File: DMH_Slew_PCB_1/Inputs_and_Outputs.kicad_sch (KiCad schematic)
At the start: 25 parts, among them J1 TS_Jack_6.35mm_Sw, J10 TS_Jack_6.35mm_Sw, J11 TS_Jack_6.35mm_Sw, J2 TS_Jack_6.35mm_Sw, J200 IDC_02x05, J3 TS_Jack_6.35mm_Sw, J4 TS_Jack_6.35mm_Sw, J5 TS_Jack_6.35mm_Sw, J6 TS_Jack_6.35mm_Sw, J7 TS_Jack_6.35mm_Sw, J8 TS_Jack_6.35mm_Sw, J9 TS_Jack_6.35mm_Sw, U1 TL074, U2 TL072

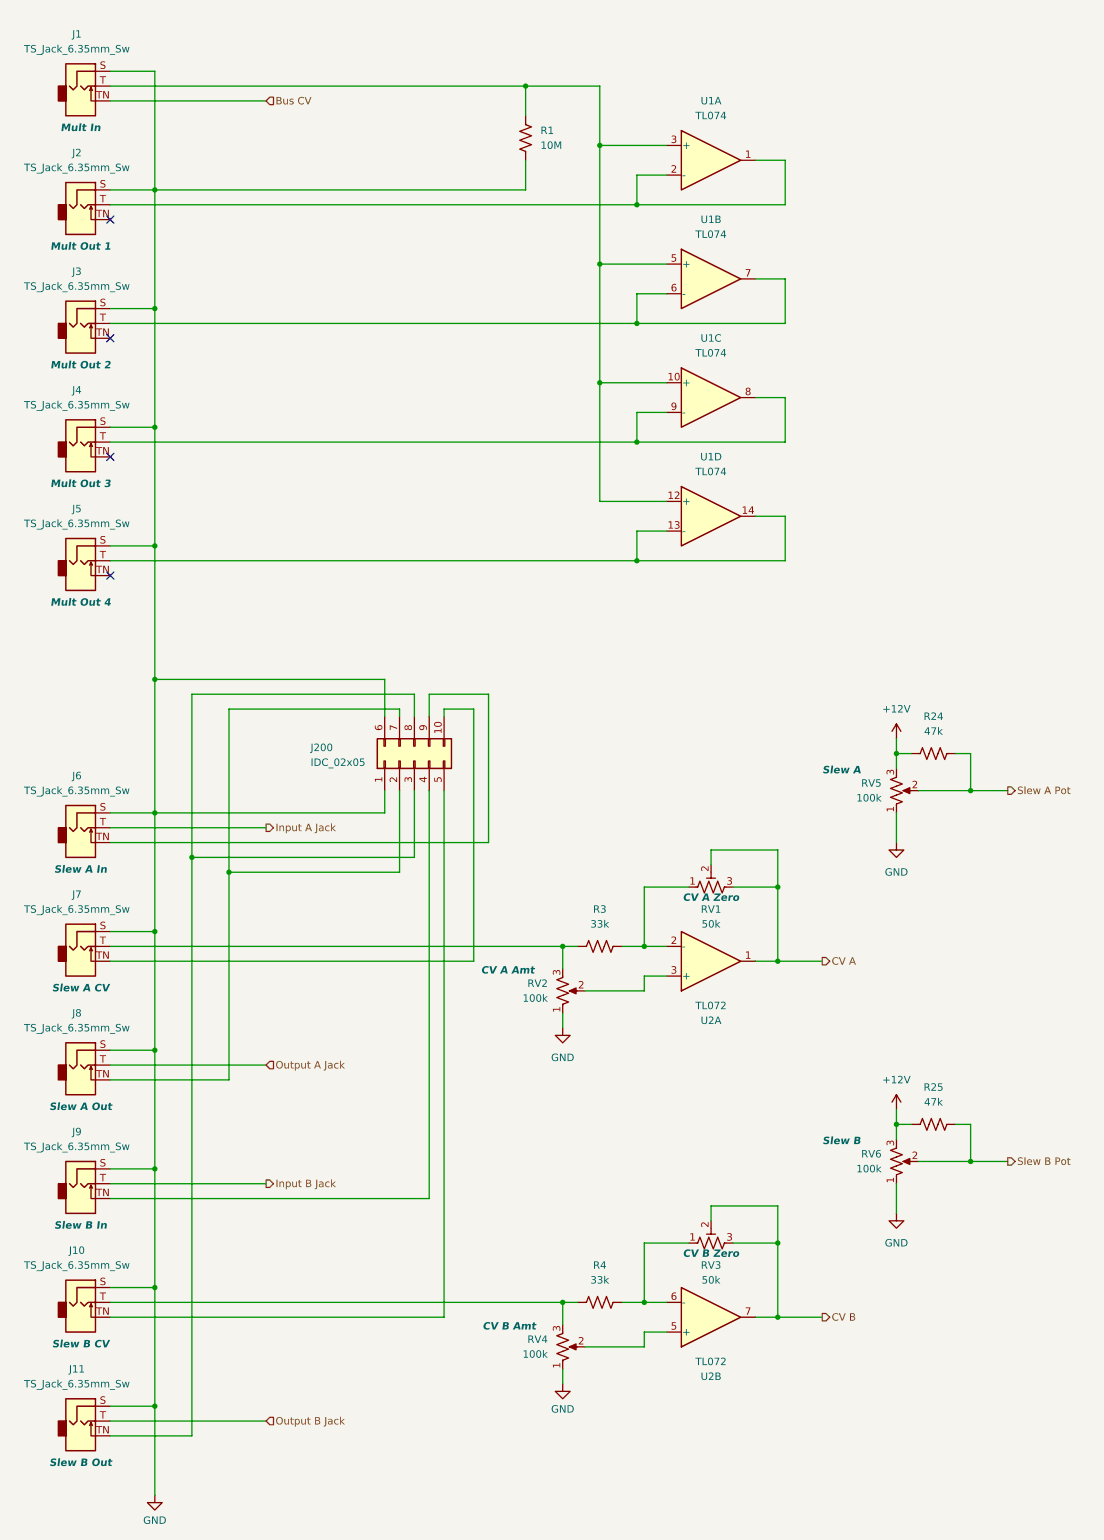
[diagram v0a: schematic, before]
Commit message: Schematic design in progress
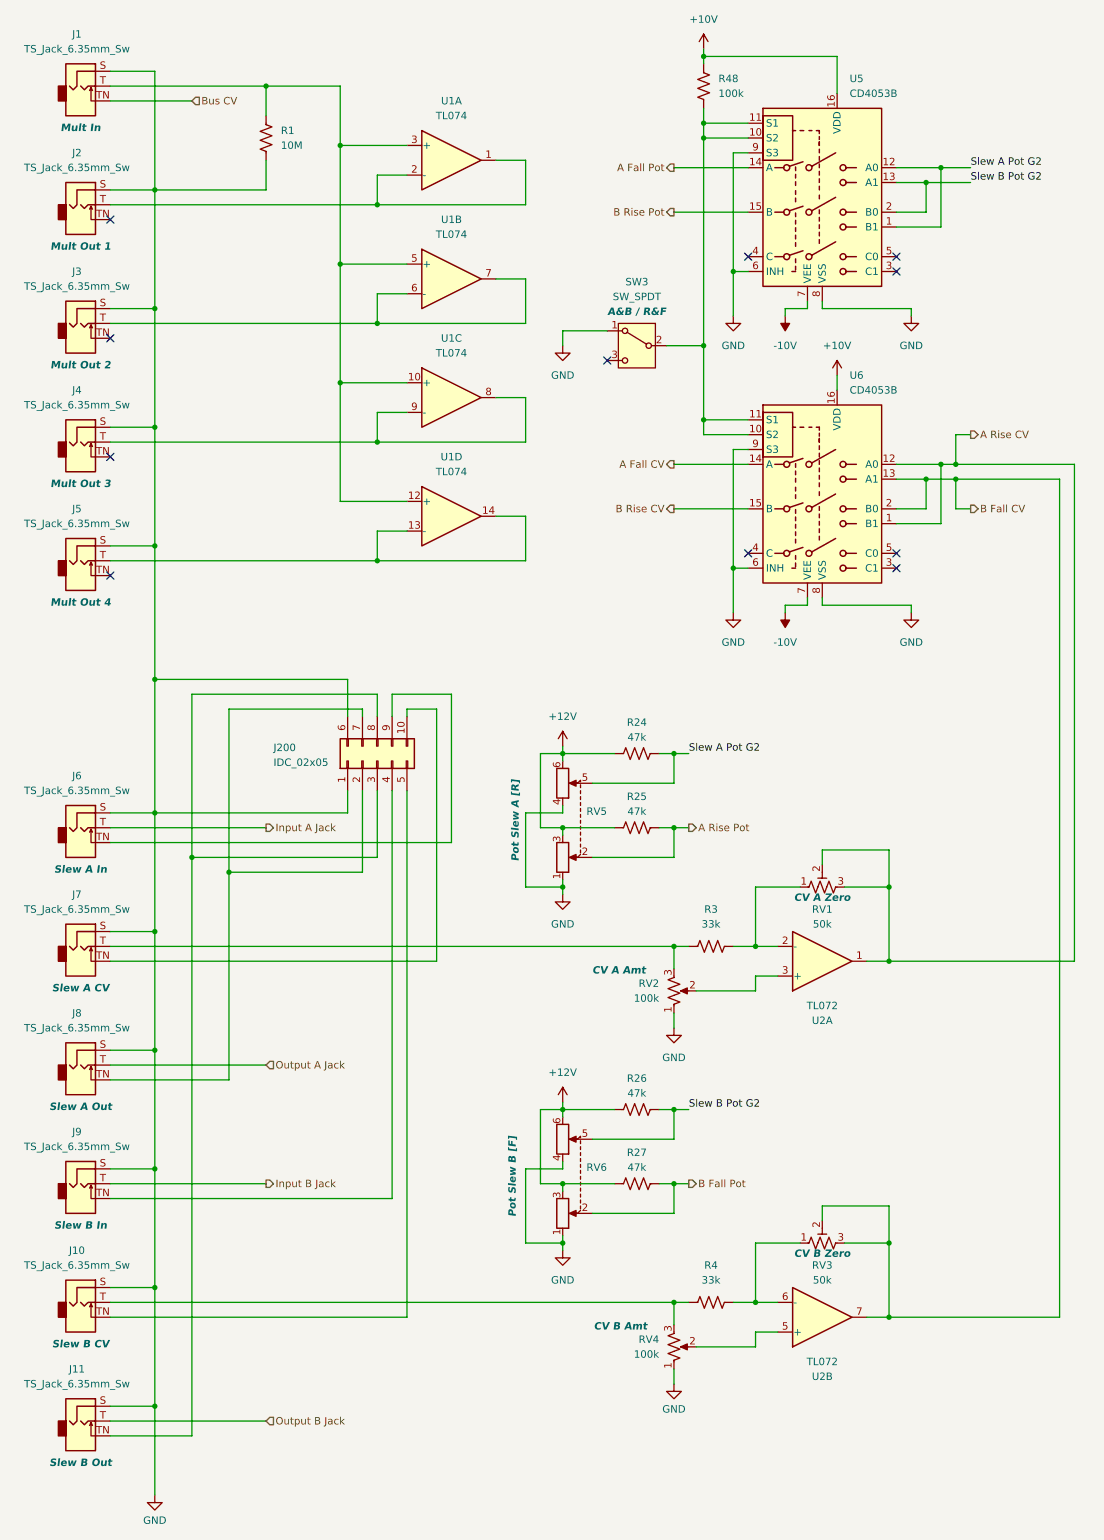
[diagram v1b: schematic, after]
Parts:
- removed RV5, RV6: 100k, SynthStuff:Potentiometer_TT_P110KH1, symbol Device:R_Potentiometer_US
- added R26, R27: 47k, Resistor_THT:R_Axial_DIN0207_L6.3mm_D2.5mm_P7.62mm_Horizontal, symbol Device:R_US
- added R48: 100k, Resistor_THT:R_Axial_DIN0207_L6.3mm_D2.5mm_P7.62mm_Horizontal, symbol Device:R_US
- added RV5, RV6: R_Potentiometer_Dual, Potentiometer_THT:Potentiometer_Alpha_RD902F-40-00D_Dual_Vertical, symbol Device:R_Potentiometer_Dual
- added SW3: SW_SPDT, symbol Switch:SW_SPDT
- added U5, U6: CD4053B, Package_DIP:DIP-16_W7.62mm_Socket, symbol Analog_Switch:CD4053B
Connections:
- net +12V: now also R26.1, R27.1, RV5.3, RV5.6, RV6.3, RV6.6
- net GND: now also RV5.1, RV5.4, RV6.1, RV6.4, SW3.1 (A), U5.6 (INH), U5.8 (VSS), U5.9 (S3), U6.6 (INH), U6.8 (VSS), U6.9 (S3)
- net CV A renamed A Rise CV
- net A Rise CV: now also U6.1 (B1), U6.12 (A0)
- net CV B renamed B Fall CV
- net B Fall CV: now also U6.13 (A1), U6.2 (B0)
- net Slew A Pot renamed Slew A Pot G2
- net Slew A Pot G2: now also RV5.5, U5.1 (B1), U5.12 (A0)
- net Slew B Pot renamed A Rise Pot
- net A Rise Pot: now also RV5.2
- new net: R48.1, SW3.2 (B), U5.10 (S2), U5.11 (S1), U6.10 (S2), U6.11 (S1)
- new net +10V: R48.2, U5.16 (VDD), U6.16 (VDD)
- new net -10V: U5.7 (VEE), U6.7 (VEE)
- new net A Fall CV: U6.14 (A)
- new net A Fall Pot: U5.14 (A)
- new net B Fall Pot: R27.2, RV6.2
- new net B Rise CV: U6.15 (B)
- new net B Rise Pot: U5.15 (B)
- new net Slew B Pot G2: R26.2, RV6.5, U5.13 (A1), U5.2 (B0)
- no-connect marks 4 -> 11
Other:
- moved on the sheet: J200, R1, R24, R3, R4, RV1, RV2, RV3, RV4, U1A, U1B, U1C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
